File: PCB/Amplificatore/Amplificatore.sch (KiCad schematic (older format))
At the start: 22 parts, among them J1 POT-1, U1 ECC83

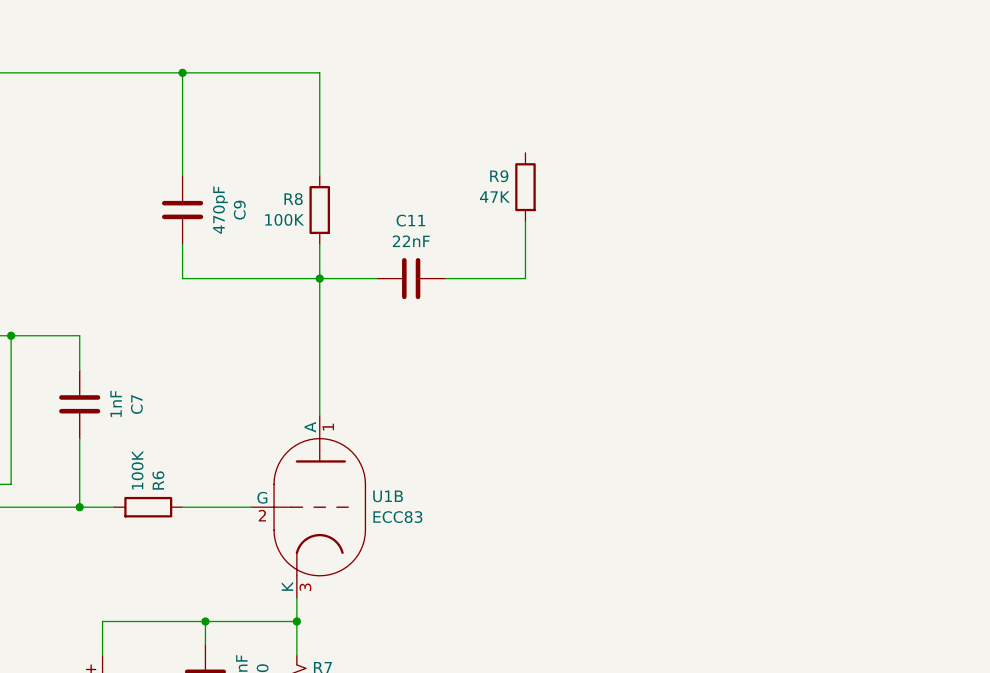
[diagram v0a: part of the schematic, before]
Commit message: Add files via upload
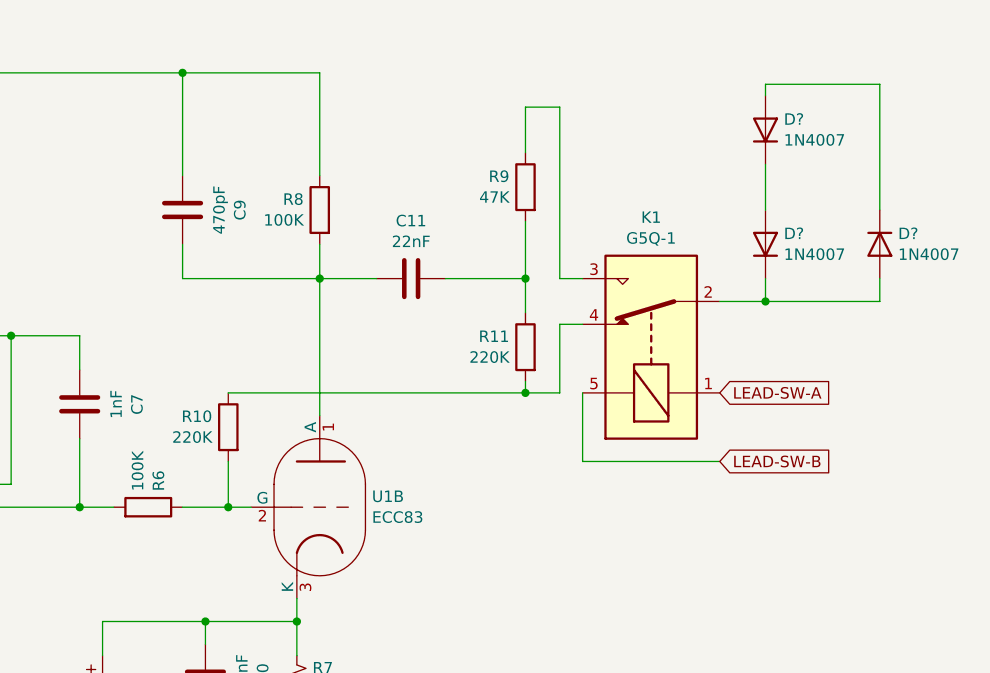
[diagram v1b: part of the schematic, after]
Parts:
- added D? (x3): 1N4007, Diode_THT:D_DO-41_SOD81_P10.16mm_Horizontal, symbol Diode:1N4007
- added K1: G5Q-1, Relay_THT:Relay_SPDT_Omron-G5Q-1, symbol Relay:G5Q-1
- added R10, R11: 220K, Resistor_SMD:R_2512_6332Metric, symbol Device:R
- J1: PN 292161-3 -> 1-292161-3
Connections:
- net at R6.1, U1.2 (G): now also R10.2
- net at C11.1, R9.2: now also R11.1
- net at R9.1: now also K1.3
- new net: D?.1 (K), D?.2 (A), K1.2
- new net: K1.4, R10.1, R11.2
- new net: D?.1 (K), D?.2 (A) (x2)
- new net LEAD-SW-A: K1.1
- new net LEAD-SW-B: K1.5
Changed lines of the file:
@@
 F 2 "Connector_PinSocket_2.00mm:PinSocket_1x03_P2.00mm_Vertical" H 4350 3900 50  0001 C CNN
 F 3 "~" H 4350 3900 50  0001 C CNN
-F 4 "292161-3" H 4350 3900 50  0001 C CNN "PN"
+F 4 "1-292161-3" H 4350 3900 50  0001 C CNN "PN"
 F 5 "M: 571-292161-3" H 4350 3900 50  0001 C CNN "FORNITORE"
 F 6 "AMP-CT, 2mm, Verticale, 3 Pin" H 4350 3900 50  0001 C CNN "NOTE"
@@
 $EndComp
 Wire Wire Line
-	5350 3900 5650 3900
+	5350 3900 5550 3900
 $Comp
 L Device:R_Small_US R7
@@
 	5350 2000 5950 2000
 Connection ~ 3200 2000
+Wire Wire Line
+	7100 3400 7100 3700
+Wire Wire Line
+	7100 3700 7700 3700
+$Comp
+L Relay:G5Q-1 K1
+U 1 1 610D4A05
+P 7400 3200
+F 0 "K1" V 7967 3200 50  0000 C CNN
+F 1 "G5Q-1" V 7876 3200 50  0000 C CNN
+F 2 "Relay_THT:Relay_SPDT_Omron-G5Q-1" H 7850 3150 50  0001 L CNN
+F 3 "https://www.omron.com/ecb/products/pdf/en-g5q.pdf" H 7400 3200 50  0001 L CNN
+F 4 "G5Q-1 DC6 " V 7400 3200 50  0001 C CNN "PN"
+F 5 "M: 653-G5Q-1DC6 " V 7400 3200 50  0001 C CNN "FORNITORE"
+	1    7400 3200
+	0    -1   -1   0
+$EndComp
+Text GLabel 7700 3400 2    50   Input ~ 0
+LEAD-SW-A
+Text GLabel 7700 3700 2    50   Input ~ 0
+LEAD-SW-B
+Connection ~ 6850 2900
+$Comp
+L Device:R R11
+U 1 1 610E3F3A
+P 6850 3200
+F 0 "R11" H 6920 3246 50  0000 L CNN
+F 1 "220K" H 6920 3155 50  0000 L CNN
+F 2 "Resistor_SMD:R_2512_6332Metric" V 6780 3200 50  0001 C CNN
+F 3 "~" H 6850 3200 50  0001 C CNN
+F 4 "CRCW2512220KJNEG " H 6850 3200 50  0001 C CNN "PN"
+F 5 "M: 71-CRCW2512J-220K-E3 " H 6850 3200 50  0001 C CNN "FORNITORE"
+F 6 "1W, 5%, 500VDC" H 6850 3200 50  0001 C CNN "NOTE"
+	1    6850 3200
+	-1   0    0    -1
+$EndComp
+$Comp
+L Device:R R10
+U 1 1 610E4EA1
+P 5550 3550
+F 0 "R10" H 5620 3596 50  0000 L CNN
+F 1 "220K" H 5620 3505 50  0000 L CNN
+F 2 "Resistor_SMD:R_2512_6332Metric" V 5480 3550 50  0001 C CNN
+F 3 "~" H 5550 3550 50  0001 C CNN
+F 4 "CRCW2512220KJNEG " H 5550 3550 50  0001 C CNN "PN"
+F 5 "M: 71-CRCW2512J-220K-E3 " H 5550 3550 50  0001 C CNN "FORNITORE"
+F 6 "1W, 5%, 500VDC" H 5550 3550 50  0001 C CNN "NOTE"
+	1    5550 3550
+	-1   0    0    -1
+$EndComp
+Wire Wire Line
+	5550 3700 5550 3900
+Connection ~ 5550 3900
+Wire Wire Line
+	5550 3900 5650 3900
+Wire Wire Line
+	5550 3400 6850 3400
+Wire Wire Line
+	6850 3400 6850 3350
+Wire Wire Line
+	6850 3050 6850 2900
+Wire Wire Line
+	6850 3400 7000 3400
+Wire Wire Line
+	7000 3400 7000 3100
+Wire Wire Line
+	7000 3100 7100 3100
+Connection ~ 6850 3400
+Wire Wire Line
+	7100 2900 7000 2900
+Wire Wire Line
+	7000 2900 7000 2150
+Wire Wire Line
+	7000 2150 6850 2150
+Wire Wire Line
+	6850 2150 6850 2350
+$Comp
+L Diode:1N4007 D?
+U 1 1 611044D8
+P 7900 2750
+F 0 "D?" V 7946 2830 50  0000 L CNN
+F 1 "1N4007" V 7855 2830 50  0000 L CNN
+F 2 "Diode_THT:D_DO-41_SOD81_P10.16mm_Horizontal" H 7900 2575 50  0001 C CNN
+F 3 "http://www.vishay.com/docs/88503/1n4001.pdf" H 7900 2750 50  0001 C CNN
+F 4 "1N4007-T" H 7900 2750 50  0001 C CNN "PN"
+F 5 "M: 621-1N4007 " H 7900 2750 50  0001 C CNN "FORNITORE"
+	1    7900 2750
+	0    1    -1   0
+$EndComp
+$Comp
+L Diode:1N4007 D?
+U 1 1 6110AC70
+P 7900 2250
+F 0 "D?" V 7946 2330 50  0000 L CNN
+F 1 "1N4007" V 7855 2330 50  0000 L CNN
+F 2 "Diode_THT:D_DO-41_SOD81_P10.16mm_Horizontal" H 7900 2075 50  0001 C CNN
+F 3 "http://www.vishay.com/docs/88503/1n4001.pdf" H 7900 2250 50  0001 C CNN
+F 4 "1N4007-T" H 7900 2250 50  0001 C CNN "PN"
+F 5 "M: 621-1N4007 " H 7900 2250 50  0001 C CNN "FORNITORE"
+	1    7900 2250
+	0    1    -1   0
+$EndComp
+Wire Wire Line
+	7900 2600 7900 2400
+$Comp
+L Diode:1N4007 D?
+U 1 1 6110D37C
+P 8400 2750
+F 0 "D?" V 8354 2830 50  0000 L CNN
+F 1 "1N4007" V 8445 2830 50  0000 L CNN
+F 2 "Diode_THT:D_DO-41_SOD81_P10.16mm_Horizontal" H 8400 2575 50  0001 C CNN
+F 3 "http://www.vishay.com/docs/88503/1n4001.pdf" H 8400 2750 50  0001 C CNN
+F 4 "1N4007-T" H 8400 2750 50  0001 C CNN "PN"
+F 5 "M: 621-1N4007 " H 8400 2750 50  0001 C CNN "FORNITORE"
+	1    8400 2750
+	0    1    1    0
+$EndComp
+Wire Wire Line
+	7900 2900 7900 3000
+Wire Wire Line
+	7900 3000 8400 3000
+Wire Wire Line
+	8400 3000 8400 2900
+Wire Wire Line
+	8400 2600 8400 2050
+Wire Wire Line
+	8400 2050 7900 2050
+Wire Wire Line
+	7900 2050 7900 2100
+Wire Wire Line
+	7700 3000 7900 3000
+Connection ~ 7900 3000
 $EndSCHEMATC
